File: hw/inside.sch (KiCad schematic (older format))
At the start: 48 parts

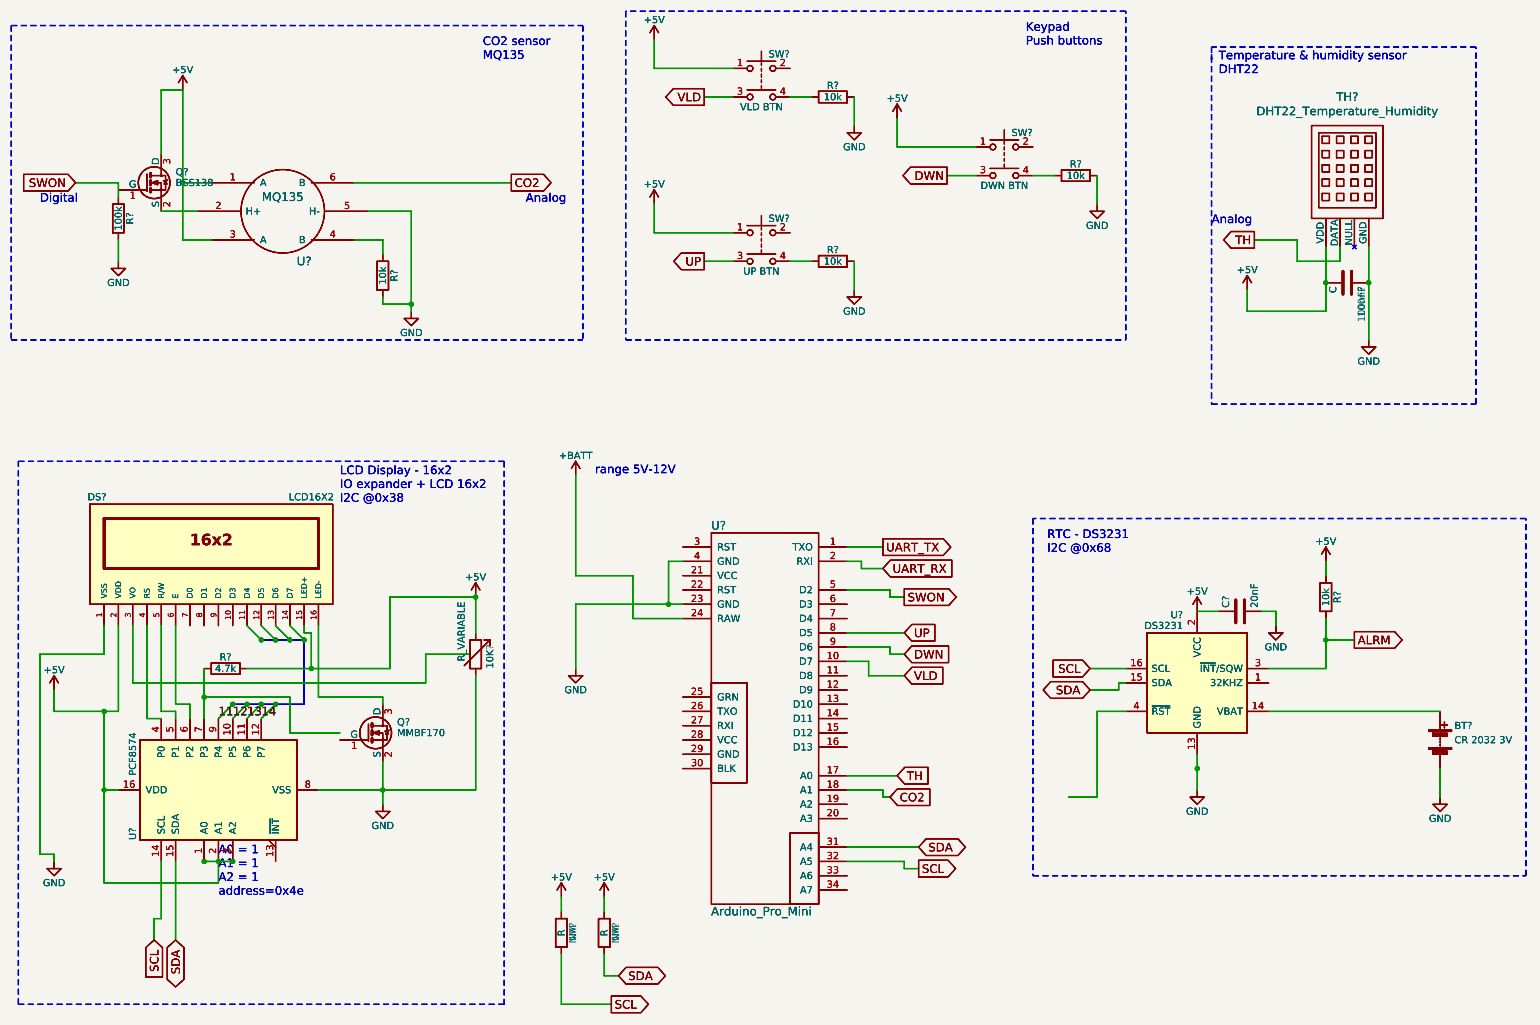
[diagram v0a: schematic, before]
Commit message: hw: annotate schematics
Signed-off-by: Pierre-Yves Kerbrat <pkerbrat@free.fr>
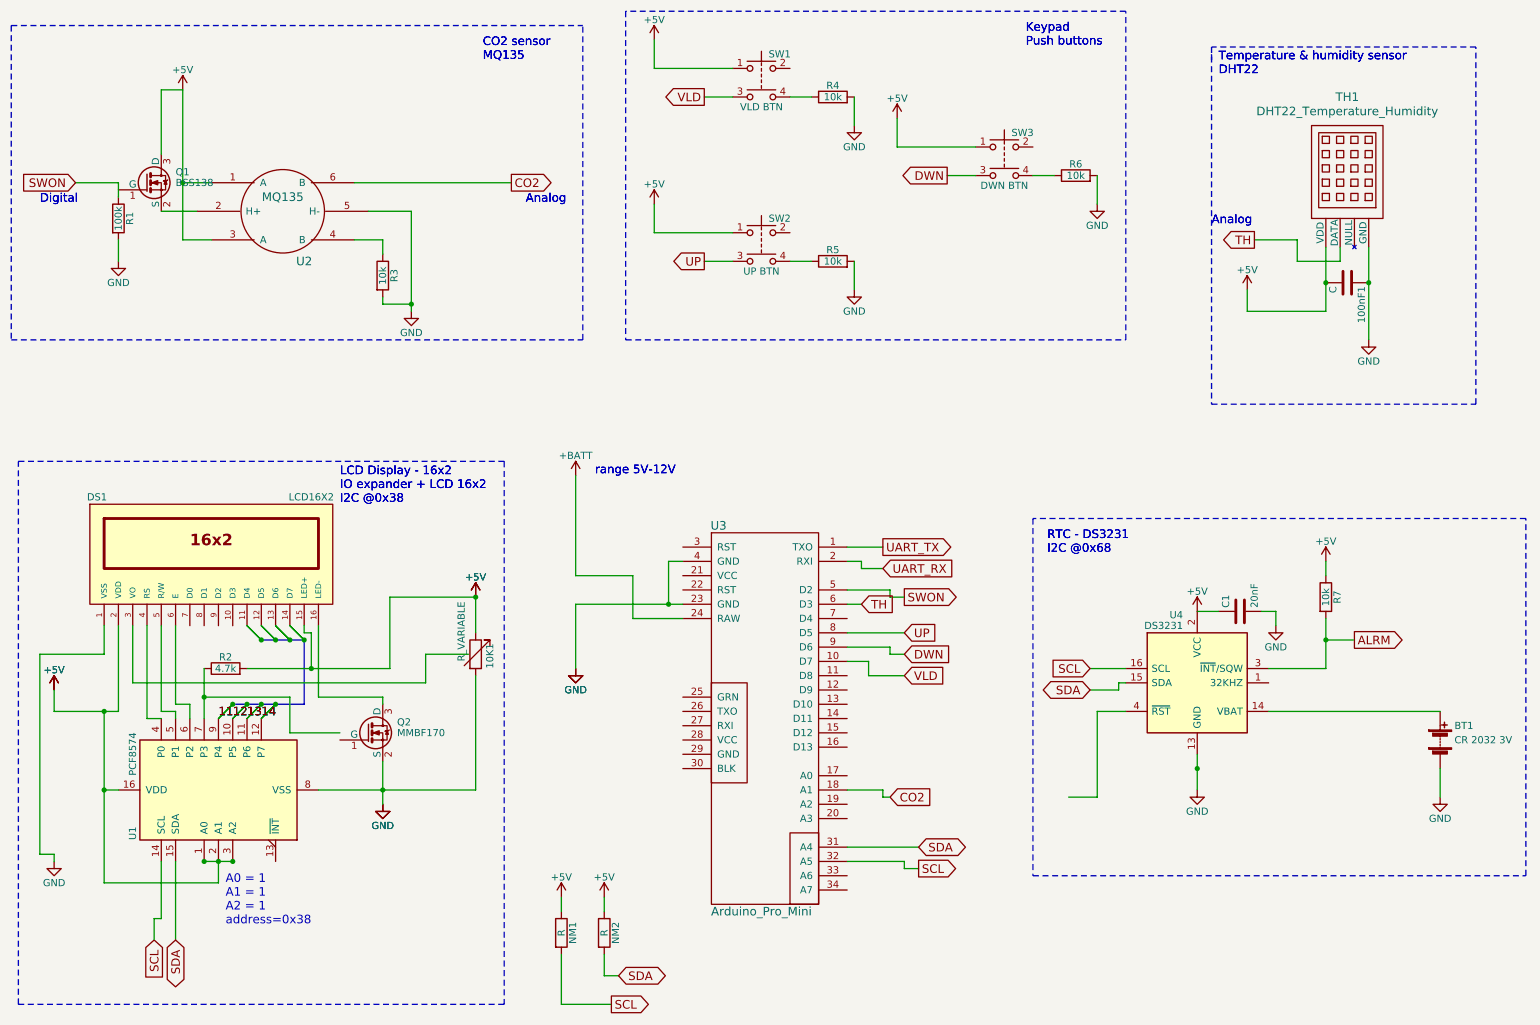
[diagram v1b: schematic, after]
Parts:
- removed 100nF: C, symbol C
- removed 10K: R_VARIABLE, symbol R_Variable
- removed BT?: CR 2032 3V, symbol Battery
- removed C?: 20nF, symbol C
- removed DS?: LCD16X2, WC1602A, symbol LCD16X2
- removed NM (x2): R, symbol R
- removed Q?: BSS138, TO_SOT_Packages_SMD:SOT-23, symbol BSS138
- removed Q?: MMBF170, TO_SOT_Packages_SMD:SOT-23, symbol MMBF170
- removed R? (x5): 10k, symbol R
- removed R?: 100k, symbol R
- removed R?: 4.7k, symbol R
- removed SW?: UP BTN, symbol SW_Push_Dual
- removed SW?: VLD BTN, symbol SW_Push_Dual
- removed SW?: DWN BTN, symbol SW_Push_Dual
- removed TH?: DHT22_Temperature_Humidity, symbol DHT22_Temperature_Humidity
- removed U?: MQ135, ~, symbol MQ135
- removed U?: PCF8574, symbol PCF8574
- removed U?: Arduino_Pro_Mini, symbol Arduino_Pro_Mini
- removed U?: DS3231, Housings_SOIC:SOIC-16_7.5x10.3mm_Pitch1.27mm, symbol DS3231
- gave numbers to parts that had none: 24
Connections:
- net TH: now also U3.6 (D3); no longer U3.17 (A0)
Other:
- note added: "A0 = 1\nA1 = 1\nA2 = 1\naddress=0x38"
- note removed: "A0 = 1\nA1 = 1\nA2 = 1\naddress=0x4e"
